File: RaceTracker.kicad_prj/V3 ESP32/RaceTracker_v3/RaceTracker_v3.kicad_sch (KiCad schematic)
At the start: 45 parts, among them J1 USB-C, J2 Battery, J3 Qwiic GPS (I2C), J4 microSD, J5 UART Debug, J6 e-Paper (steckbar) 8p, SW1 PWR, SW2 RESET, SW3 BOOT, U1 ESP32-S3-WROOM-1-N8, U2 MCP73831T-2ACI/OT, U3 AP2112K-3.3, U4 WSEN-ISDS

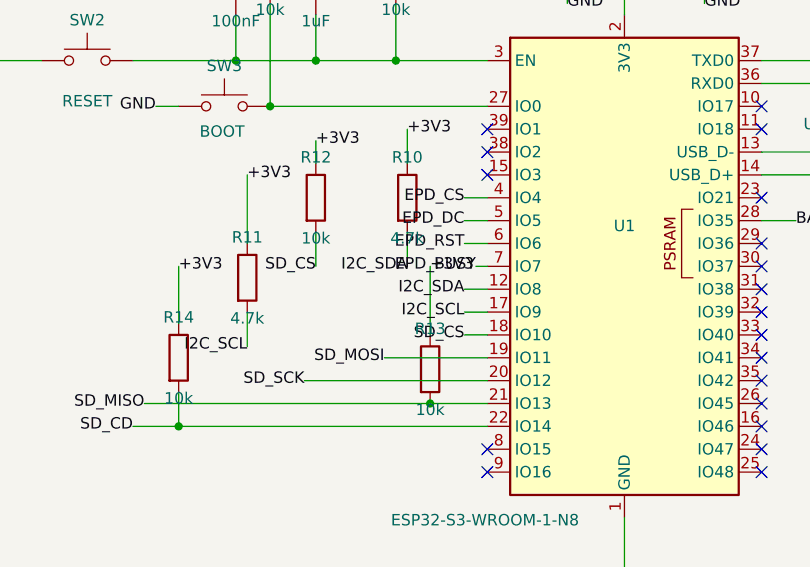
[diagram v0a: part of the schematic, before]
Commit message: V3: GND/+3V3 Planes, Power-Routing, Teilrouting der Signalnetze
Co-Authored-By: Claude Sonnet 5 <noreply@anthropic.com>
Claude-Session: https://claude.ai/code/session_01KJ1x8W8LsYuDo52VfB14br
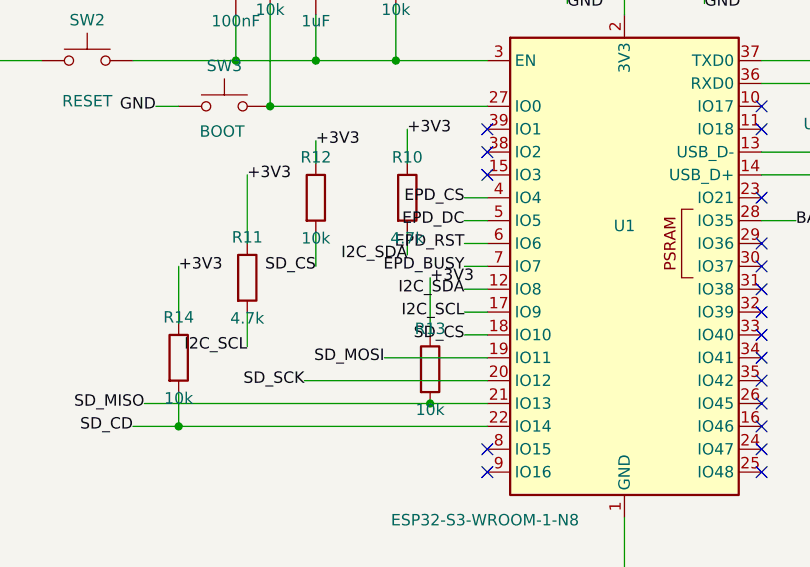
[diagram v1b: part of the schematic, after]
